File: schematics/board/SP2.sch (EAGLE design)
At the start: 15 parts

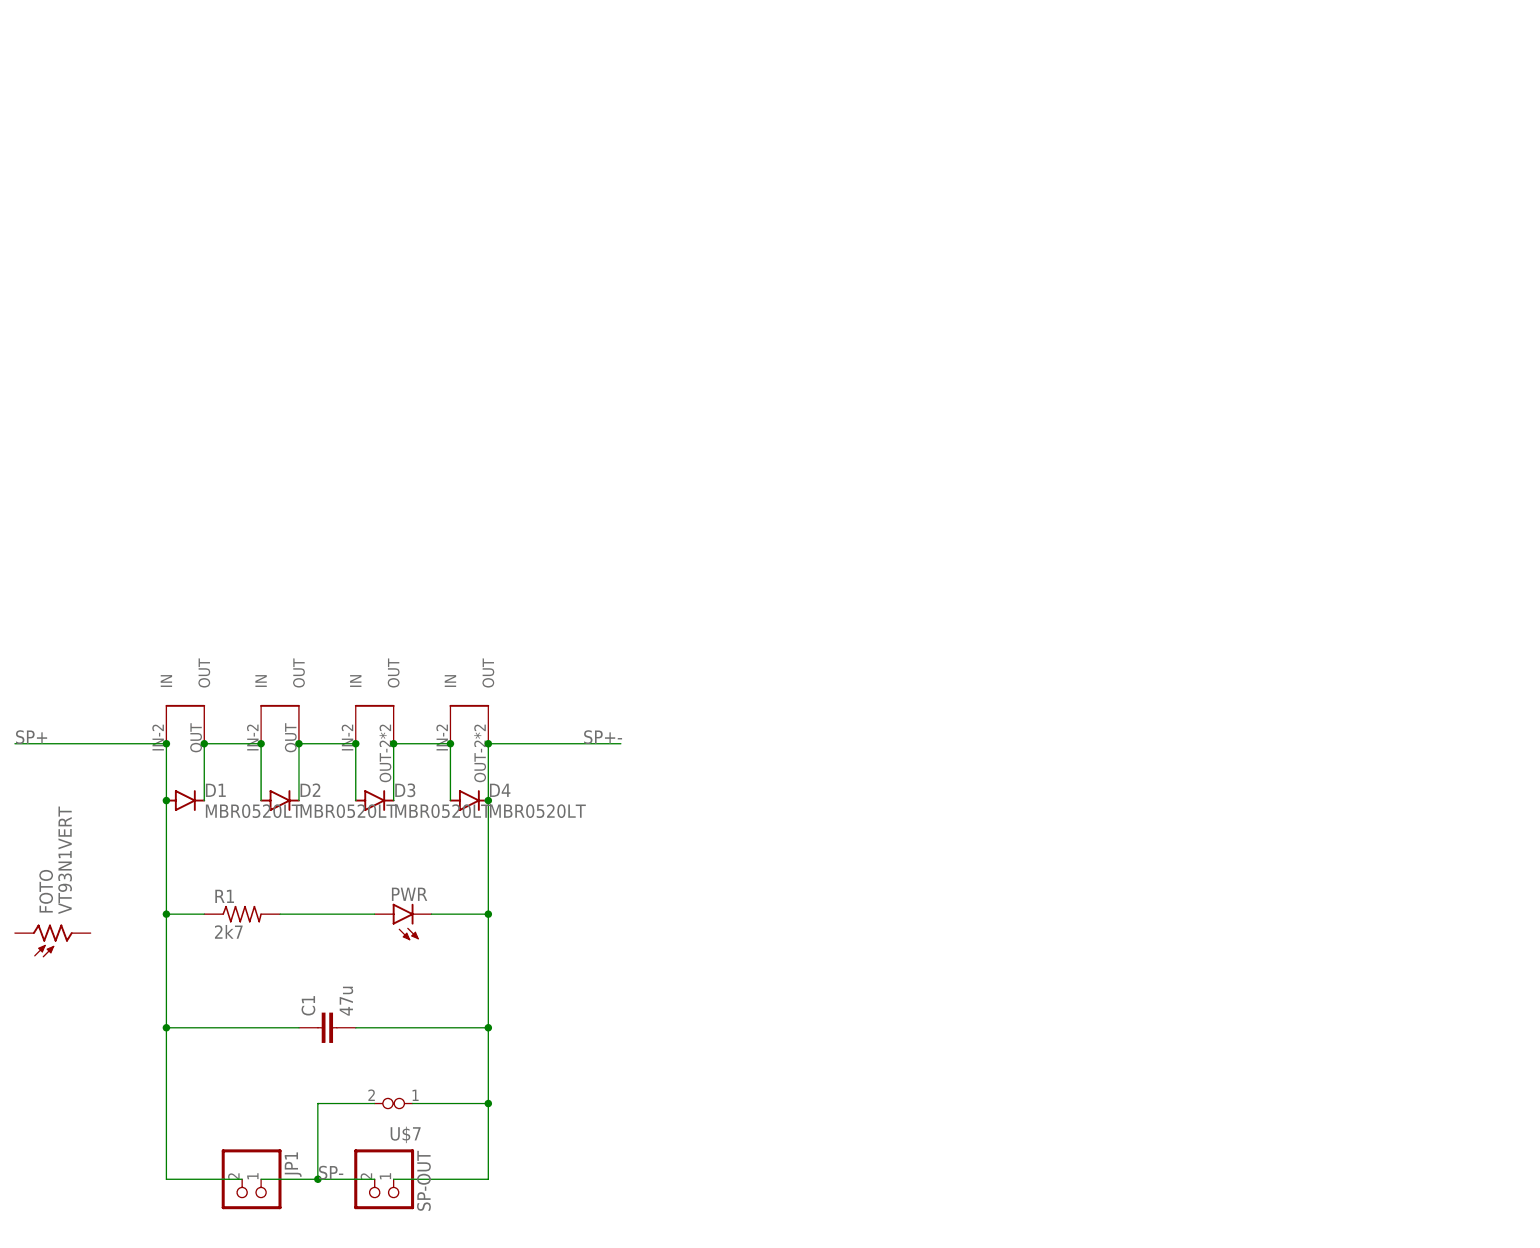
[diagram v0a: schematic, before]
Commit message: ПЛАТЫ, АААААААААААААААААААААААААААА
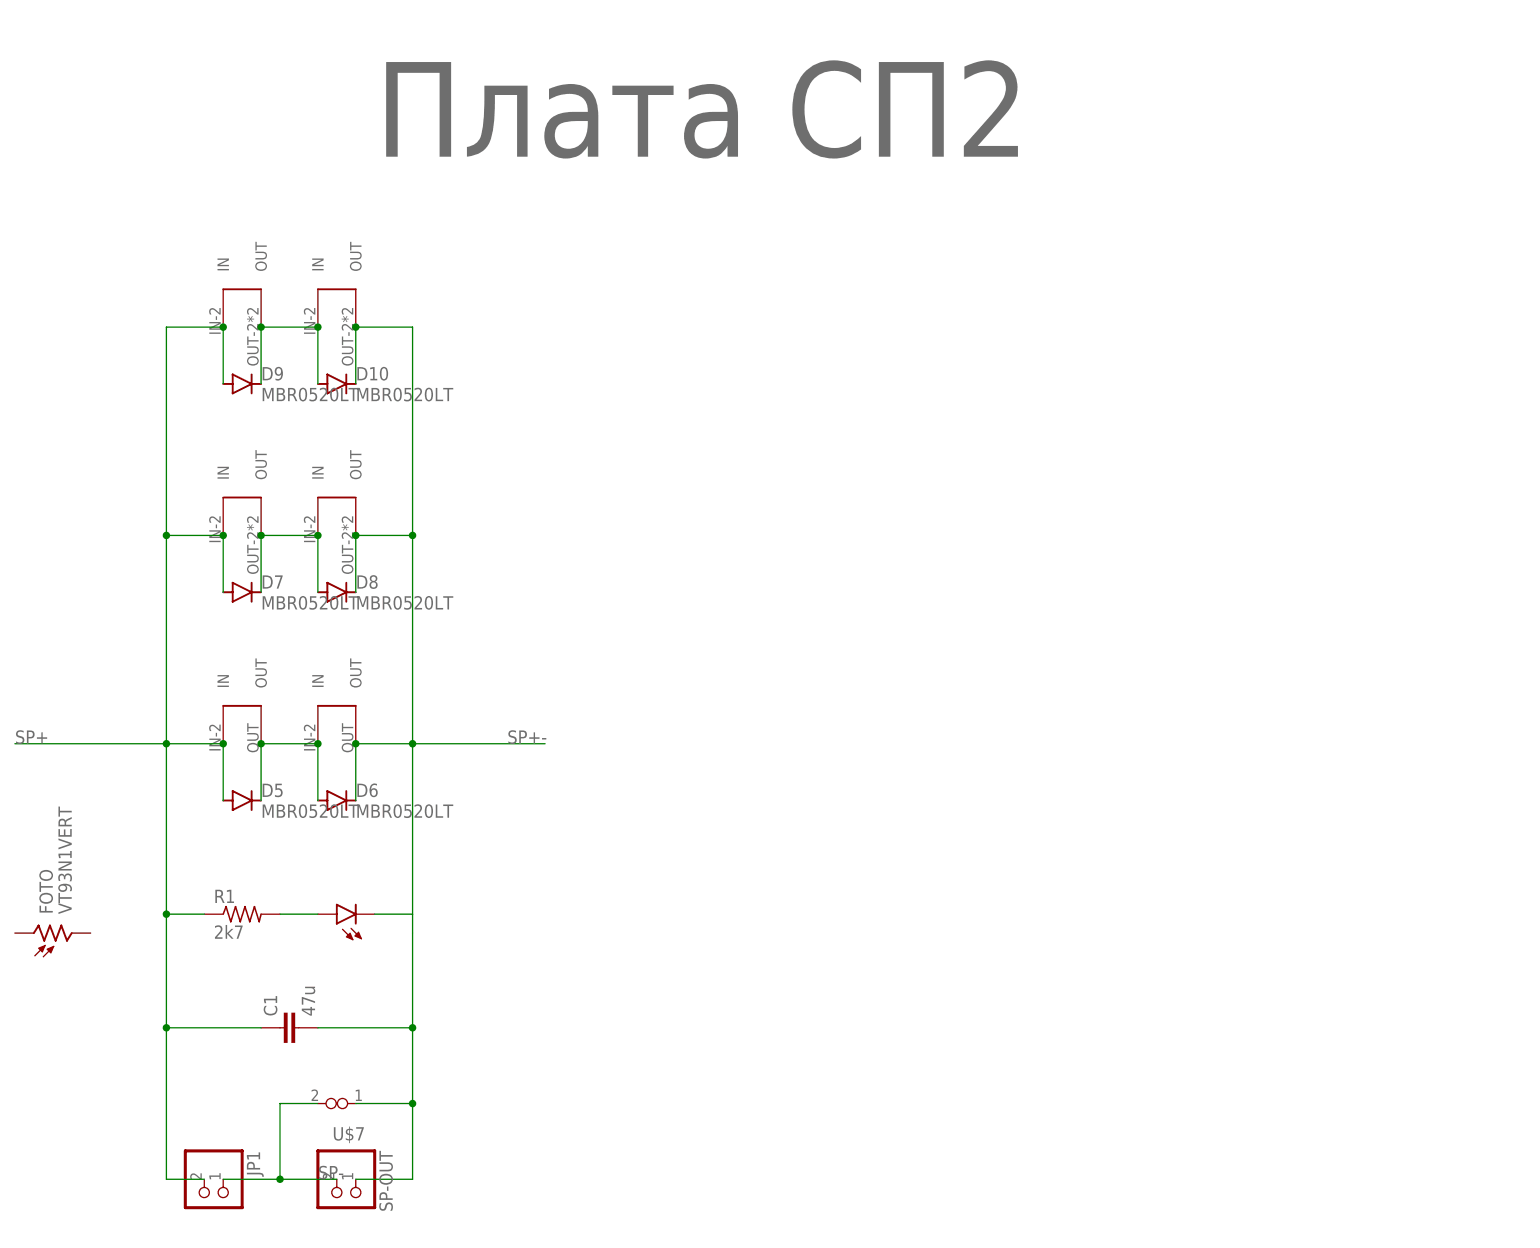
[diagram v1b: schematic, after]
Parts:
- removed D1, D2, D3, D4: MBR0520LT, diode:MBR0520LT
- removed U$2: SOLAR-2_1, KNPN-2023:SOLAR-2_1
- removed U$3, U$4: SOLAR-2_0, KNPN-2023:SOLAR-2_0
- added D10, D5, D6, D7, D8, D9: MBR0520LT, diode:MBR0520LT
- added U$10, U$11, U$8, U$9: SOLAR-2_0, CanCubeSat:SOLAR-2_0
- added U$5, U$6: SOLAR-2_1, CanCubeSat:SOLAR-2_1
- U$1: value SOLAR-2_1 -> Плата СП2; device KNPN-2023:SOLAR-2_1 -> UNKNOWN-2024:LOGOPCB-""
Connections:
- removed net N$1: D1.C, D2.A, U$1.OUT, U$2.IN
- removed net N$2: D2.C, D3.A, U$2.OUT, U$3.IN
- removed net N$3: D3.C, D4.A, U$3.OUT, U$4.IN
- new net N$5: D5.C, D6.A, U$5.OUT, U$6.IN
- new net N$7: D7.C, D8.A, U$8.OUT, U$9.IN
- new net N$8: D10.A, D9.C, U$10.OUT, U$11.IN
- net SP+: now also D5.A, D7.A, D9.A, U$10.IN, U$5.IN, U$8.IN; no longer D1.A, U$1.IN
- net SP+-: now also D10.C, D6.C, D8.C, U$11.OUT, U$6.OUT, U$9.OUT; no longer D4.C, U$4.OUT
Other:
- moved on the sheet: C1, JP1, SP-OUT, U$7
